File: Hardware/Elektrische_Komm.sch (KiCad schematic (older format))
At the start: 133 parts, among them J1 Conn_01x01, J2 Conn_01x01, J3 Conn_01x01, J4 Conn_01x04, J5 USB_OTG, Q1 BSZ014NE2LS5IF, Q10 BSR202NL6327HTSA1, Q11 BSR202NL6327HTSA1, Q12 BSR202NL6327HTSA1, Q13 BSR202NL6327HTSA1, Q14 BSR202NL6327HTSA1, Q2 BSZ014NE2LS5IF, Q3 BSZ014NE2LS5IF, Q4 BSZ014NE2LS5IF, Q5 BSZ014NE2LS5IF, Q6 BSZ014NE2LS5IF, Q7 BSR202NL6327HTSA1, Q8 BSR202NL6327HTSA1, Q9 BSR202NL6327HTSA1, SW1 SW_Push, SW2 SW_Push, U1 TS374IDT, U10 TPS561201, U11 LVM339IDT, U12 STM32F413R(G-H)Tx_u, U2 UCC27710, U3 ACS723LLCTR, U4 UCC27710, U5 ACS723LLCTR, U6 UCC27710, U7 74HC32D, U8 74LVC2G02, U9 LDK715M50R, Y1 10MHz

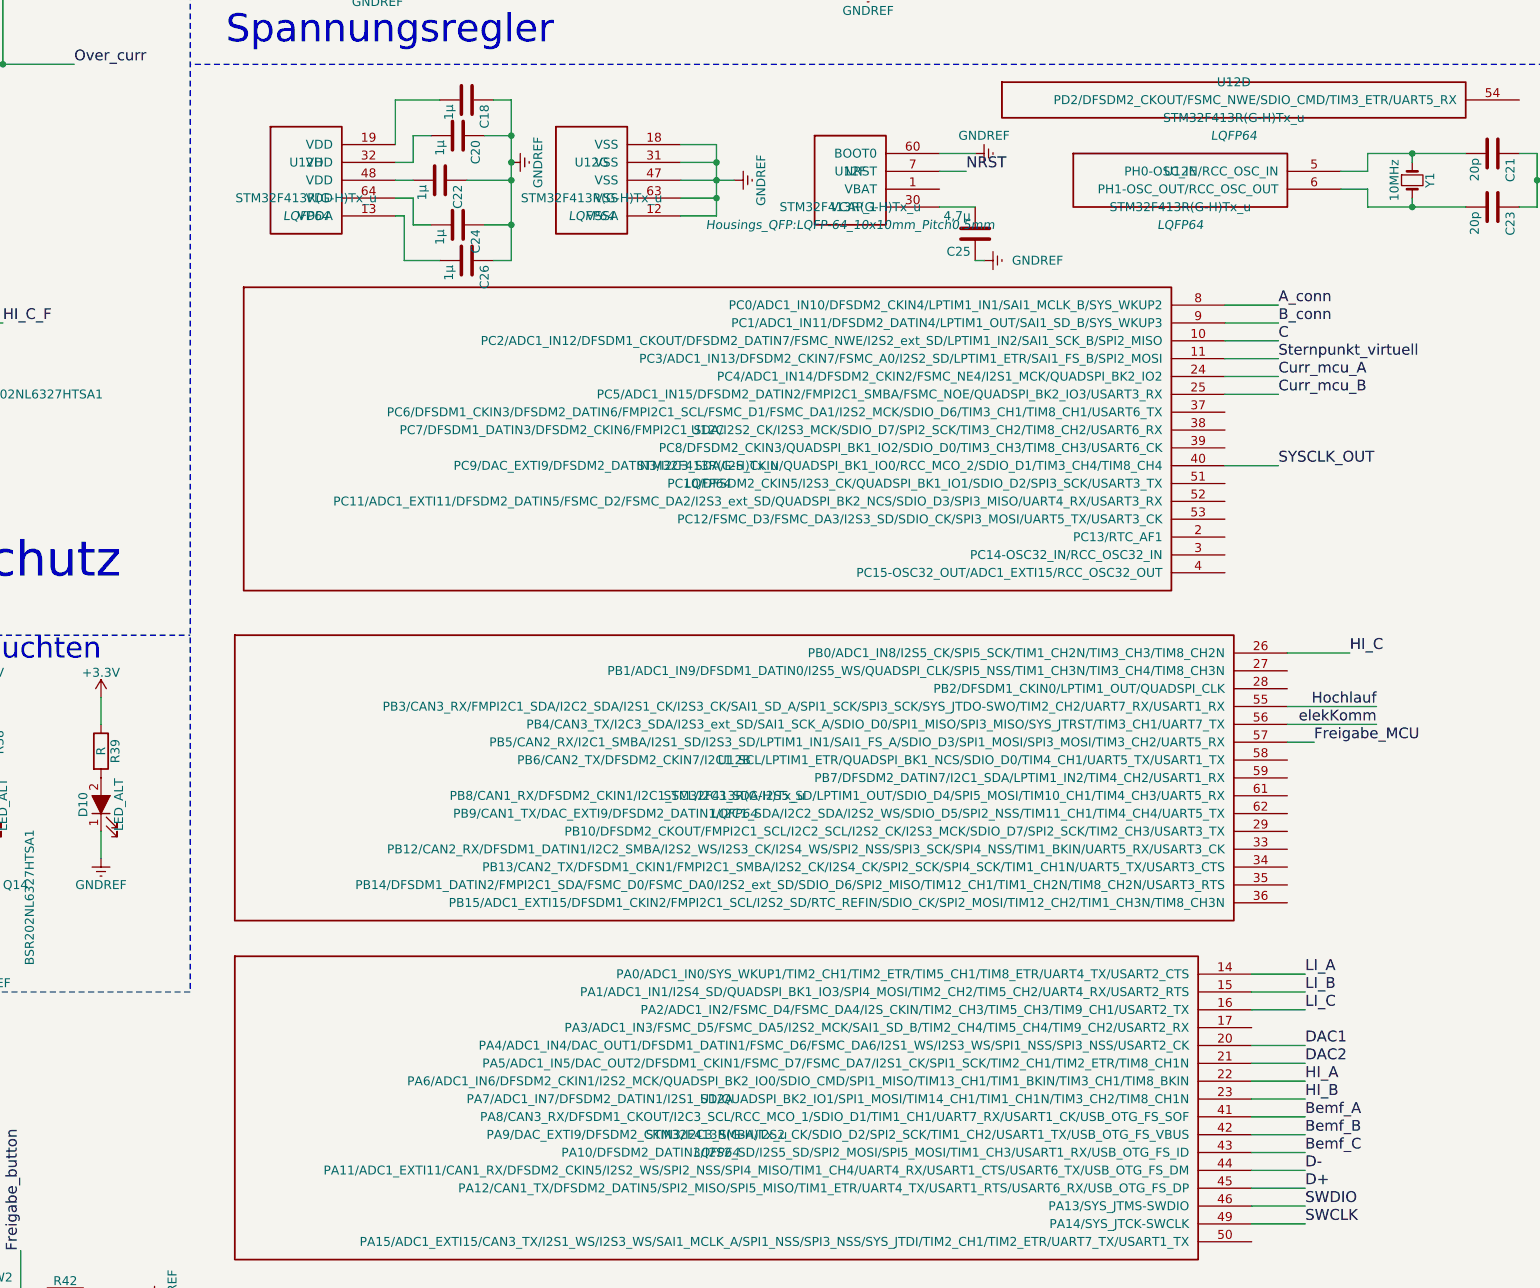
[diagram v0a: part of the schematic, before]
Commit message: Schematic fertig
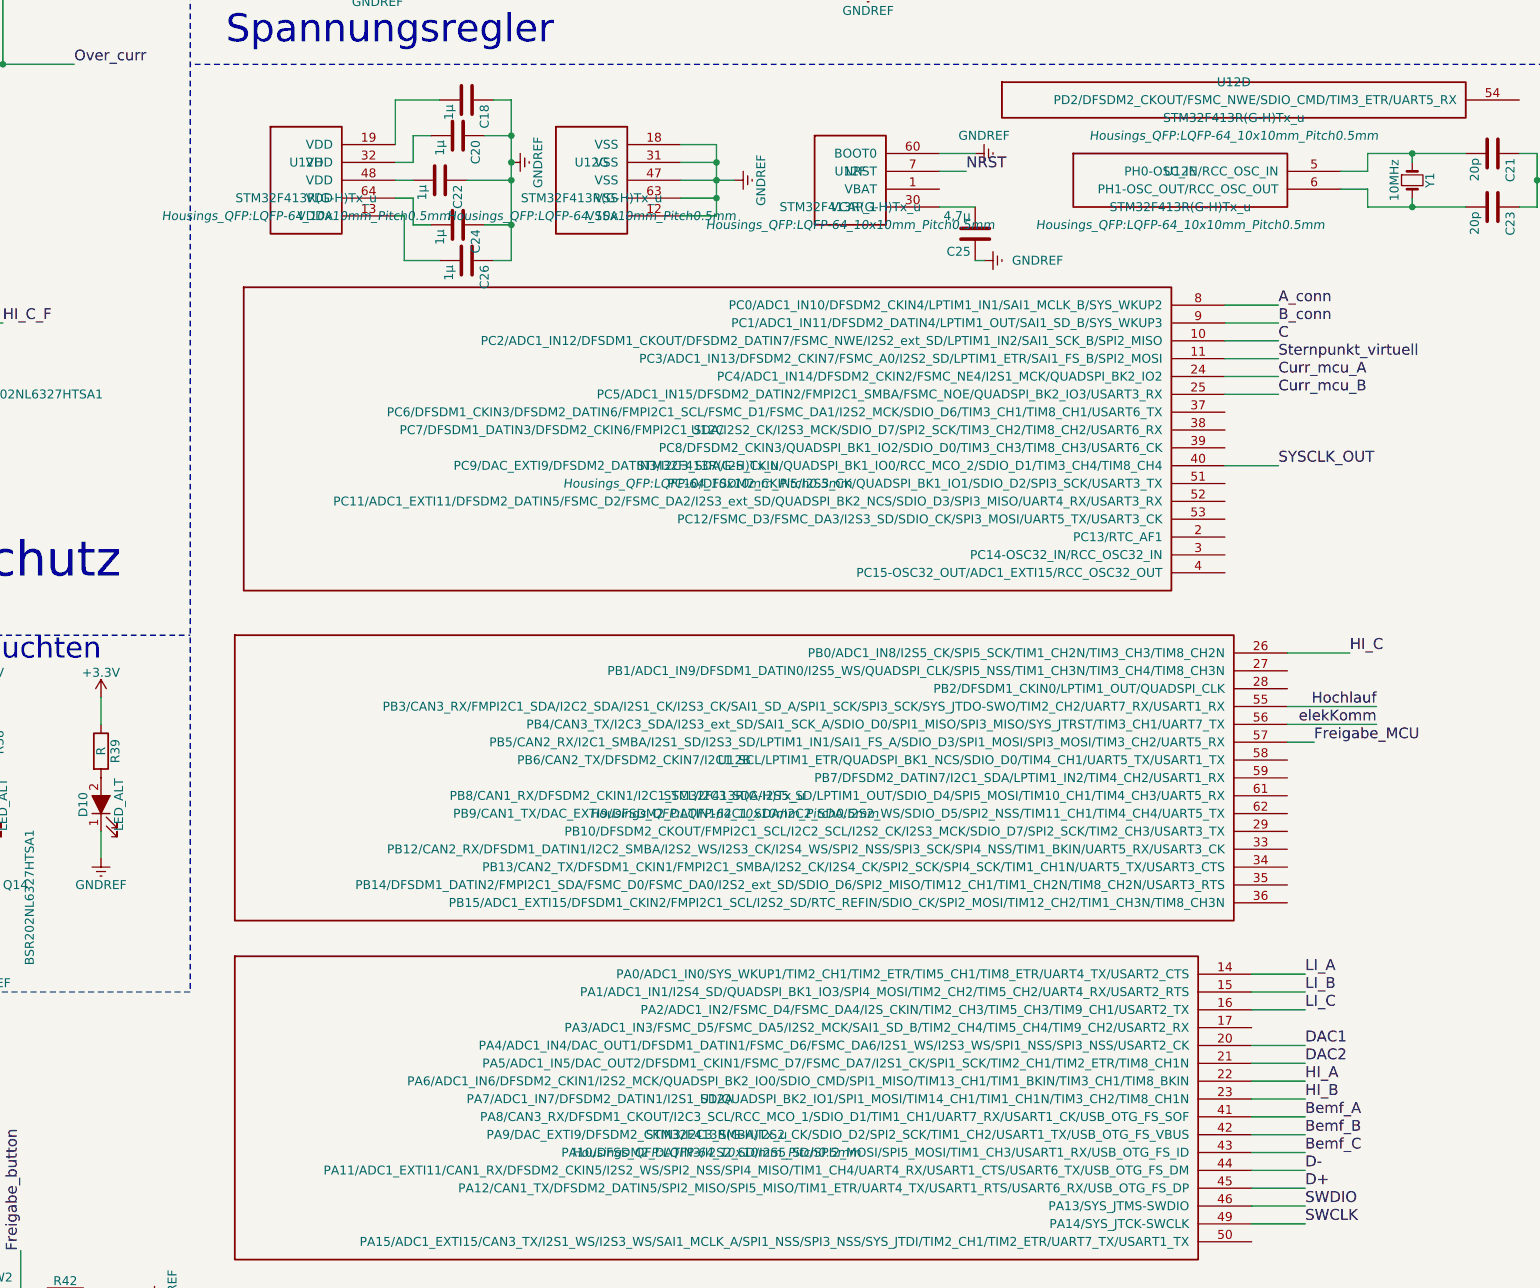
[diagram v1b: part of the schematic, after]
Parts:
- C19: footprint (none) -> Capacitors_SMD:C_0603
- D10, D8, D9: footprint (none) -> LEDs:LED_0805
- D6, D7: footprint (none) -> LEDs:LED_0805_HandSoldering
- U12: footprint LQFP64 -> Housings_QFP:LQFP-64_10x10mm_Pitch0.5mm
- U7: footprint (none) -> Housings_SSOP:TSSOP-14_4.4x5mm_Pitch0.65mm
- U8: footprint (none) -> Housings_SSOP:TSSOP-8_3x3mm_Pitch0.65mm
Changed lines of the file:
@@
 F 0 "U8" H 8950 8050 60  0000 C CNN
 F 1 "74LVC2G02" H 8950 7950 60  0000 C CNN
-F 2 "" H 8950 8150 60  0001 C CNN
+F 2 "Housings_SSOP:TSSOP-8_3x3mm_Pitch0.65mm" H 8950 8150 60  0001 C CNN
 F 3 "" H 8950 8150 60  0001 C CNN
 	2    8950 8150
@@
 F 0 "C19" H 8475 8350 50  0000 L CNN
 F 1 "100n" H 8475 8150 50  0000 L CNN
-F 2 "" H 8488 8100 50  0001 C CNN
+F 2 "Capacitors_SMD:C_0603" H 8488 8100 50  0001 C CNN
 F 3 "" H 8450 8250 50  0001 C CNN
 	1    8450 8250
@@
 F 0 "U7" H 4100 7050 60  0000 C CNN
 F 1 "74HC32D" H 4200 6950 60  0000 C CNN
-F 2 "" H 3850 7150 60  0001 C CNN
+F 2 "Housings_SSOP:TSSOP-14_4.4x5mm_Pitch0.65mm" H 3850 7150 60  0001 C CNN
 F 3 "" H 3850 7150 60  0001 C CNN
 	2    3850 7150
@@
 F 0 "U7" H 4050 11250 60  0000 C CNN
 F 1 "74HC32D" H 4000 11150 60  0000 C CNN
-F 2 "" H 4000 11350 60  0001 C CNN
+F 2 "Housings_SSOP:TSSOP-14_4.4x5mm_Pitch0.65mm" H 4000 11350 60  0001 C CNN
 F 3 "" H 4000 11350 60  0001 C CNN
 	4    4000 11350
@@
 F 0 "U7" H 7000 6800 60  0000 C CNN
 F 1 "74HC32D" H 6950 6700 60  0000 C CNN
-F 2 "" H 6950 6900 60  0001 C CNN
+F 2 "Housings_SSOP:TSSOP-14_4.4x5mm_Pitch0.65mm" H 6950 6900 60  0001 C CNN
 F 3 "" H 6950 6900 60  0001 C CNN
 	1    6950 6900
@@
 F 0 "U7" H 5900 8250 60  0000 C CNN
 F 1 "74HC32D" H 5850 8150 60  0000 C CNN
-F 2 "" H 5850 8350 60  0001 C CNN
+F 2 "Housings_SSOP:TSSOP-14_4.4x5mm_Pitch0.65mm" H 5850 8350 60  0001 C CNN
 F 3 "" H 5850 8350 60  0001 C CNN
 	3    5850 8350
@@
 F 0 "D7" H 8150 12100 50  0000 C CNN
 F 1 "LED_ALT" H 8150 11900 50  0000 C CNN
-F 2 "" H 8150 12000 50  0001 C CNN
+F 2 "LEDs:LED_0805_HandSoldering" H 8150 12000 50  0001 C CNN
 F 3 "" H 8150 12000 50  0001 C CNN
 	1    8150 12000
@@
 F 0 "D6" H 7350 12100 50  0000 C CNN
 F 1 "LED_ALT" H 7350 11900 50  0000 C CNN
-F 2 "" H 7350 12000 50  0001 C CNN
+F 2 "LEDs:LED_0805_HandSoldering" H 7350 12000 50  0001 C CNN
 F 3 "" H 7350 12000 50  0001 C CNN
 	1    7350 12000
@@
 F 0 "D8" H 8900 12100 50  0000 C CNN
 F 1 "LED_ALT" H 8900 11900 50  0000 C CNN
-F 2 "" H 8900 12000 50  0001 C CNN
+F 2 "LEDs:LED_0805" H 8900 12000 50  0001 C CNN
 F 3 "" H 8900 12000 50  0001 C CNN
 	1    8900 12000
@@
 F 0 "D9" H 9650 12100 50  0000 C CNN
 F 1 "LED_ALT" H 9650 11900 50  0000 C CNN
-F 2 "" H 9650 12000 50  0001 C CNN
+F 2 "LEDs:LED_0805" H 9650 12000 50  0001 C CNN
 F 3 "" H 9650 12000 50  0001 C CNN
 	1    9650 12000
@@
 F 0 "D10" H 10300 12100 50  0000 C CNN
 F 1 "LED_ALT" H 10300 11900 50  0000 C CNN
-F 2 "" H 10300 12000 50  0001 C CNN
+F 2 "LEDs:LED_0805" H 10300 12000 50  0001 C CNN
 F 3 "" H 10300 12000 50  0001 C CNN
 	1    10300 12000
@@
 F 0 "U12" H 13850 11950 50  0000 C CNN
 F 1 "STM32F413R(G-H)Tx_u" H 13850 11750 50  0000 C CNN
-F 2 "LQFP64" H 13850 11650 50  0000 C CIN
+F 2 "Housings_QFP:LQFP-64_10x10mm_Pitch0.5mm" H 13850 11650 50  0000 C CIN
 F 3 "" H 13850 11850 50  0000 C CNN
 	2    13850 11850
@@
 F 0 "U12" H 13700 10100 50  0000 C CNN
 F 1 "STM32F413R(G-H)Tx_u" H 13700 9900 50  0000 C CNN
-F 2 "LQFP64" H 13700 9800 50  0000 C CIN
+F 2 "Housings_QFP:LQFP-64_10x10mm_Pitch0.5mm" H 13700 9800 50  0000 C CIN
 F 3 "" H 13700 10000 50  0000 C CNN
 	3    13700 10000
@@
 F 0 "U12" H 16650 8150 50  0000 C CNN
 F 1 "STM32F413R(G-H)Tx_u" H 16650 7950 50  0000 C CNN
-F 2 "LQFP64" H 16650 7850 50  0000 C CIN
+F 2 "Housings_QFP:LQFP-64_10x10mm_Pitch0.5mm" H 16650 7850 50  0000 C CIN
 F 3 "" H 16650 8050 50  0000 C CNN
 	4    16650 8050
@@
 F 0 "U12" H 16350 8650 50  0000 C CNN
 F 1 "STM32F413R(G-H)Tx_u" H 16350 8450 50  0000 C CNN
-F 2 "LQFP64" H 16350 8350 50  0000 C CIN
+F 2 "Housings_QFP:LQFP-64_10x10mm_Pitch0.5mm" H 16350 8350 50  0000 C CIN
 F 3 "" H 16350 8550 50  0000 C CNN
 	5    16350 8550
@@
 F 0 "U12" H 13750 13850 50  0000 C CNN
 F 1 "STM32F413R(G-H)Tx_u" H 13750 13650 50  0000 C CNN
-F 2 "LQFP64" H 13750 13550 50  0000 C CIN
+F 2 "Housings_QFP:LQFP-64_10x10mm_Pitch0.5mm" H 13750 13550 50  0000 C CIN
 F 3 "" H 13750 13750 50  0000 C CNN
 	1    13750 13750
@@
 F 0 "U12" H 13050 8600 50  0000 C CNN
 F 1 "STM32F413R(G-H)Tx_u" H 13050 8400 50  0000 C CNN
-F 2 "LQFP64" H 13050 8300 50  0000 C CIN
+F 2 "Housings_QFP:LQFP-64_10x10mm_Pitch0.5mm" H 13050 8300 50  0000 C CIN
 F 3 "" H 13050 8500 50  0000 C CNN
 	7    13050 8500
@@
 F 0 "U12" H 11450 8600 50  0000 C CNN
 F 1 "STM32F413R(G-H)Tx_u" H 11450 8400 50  0000 C CNN
-F 2 "LQFP64" H 11450 8300 50  0000 C CIN
+F 2 "Housings_QFP:LQFP-64_10x10mm_Pitch0.5mm" H 11450 8300 50  0000 C CIN
 F 3 "" H 11450 8500 50  0000 C CNN
 	8    11450 8500
